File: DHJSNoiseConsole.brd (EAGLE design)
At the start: 88.9 x 34 mm, 11 parts

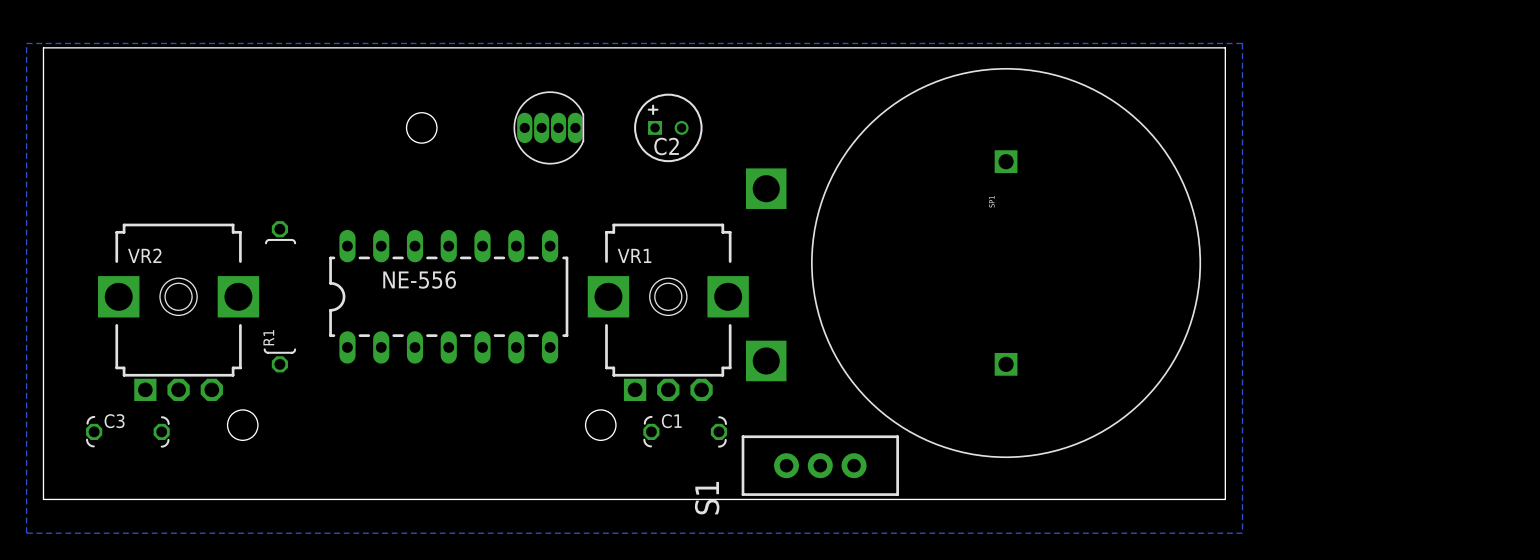
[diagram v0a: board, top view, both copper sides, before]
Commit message: board
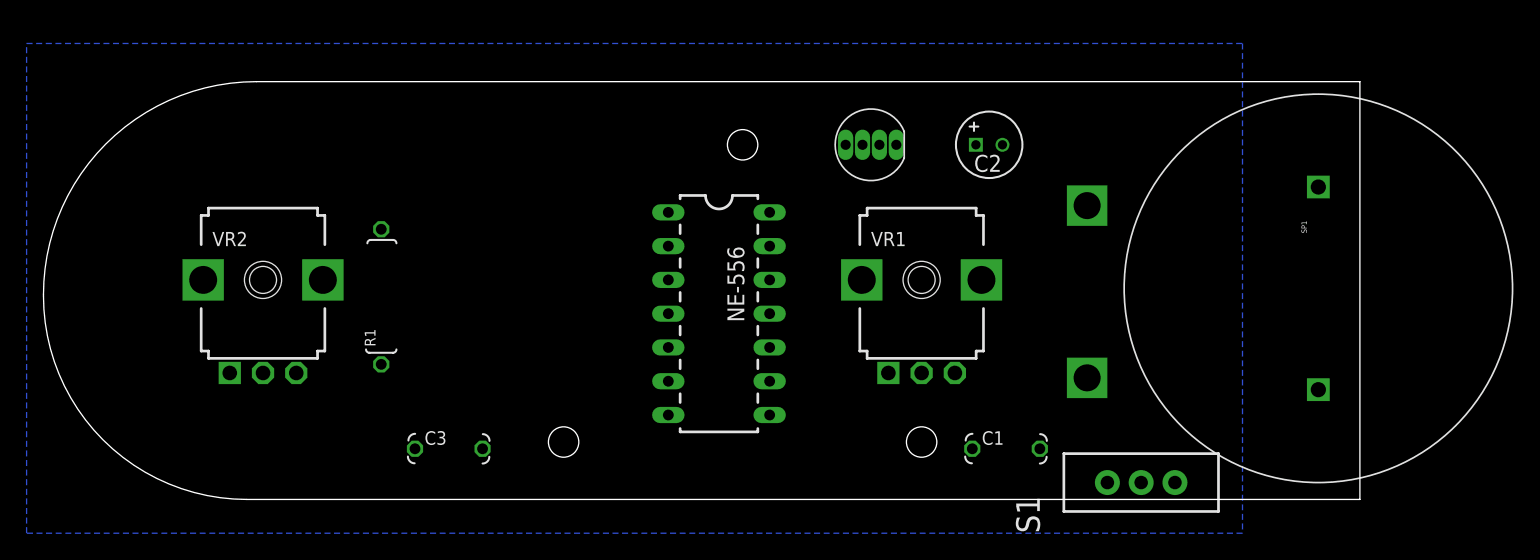
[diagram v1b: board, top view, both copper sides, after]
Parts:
- moved C1 24.2 mm to (72.4, 3.81)
- moved C2 24.2 mm to (71.1, 26.7)
- moved C3 24.2 mm to (30.5, 3.81)
- moved BAT1 24.2 mm to (25.4, 30.5)
- moved D1 24.2 mm to (62.2, 26.7)
- moved S1 24.2 mm to (82.5, 1.27)
- moved SP1 23.6 mm to (95.9, 15.9)
- moved NE-556 19.2 mm to (50.8, 12.7), turned to 270 degrees
- moved VR1 19.1 mm to (66.0, 16.5)
- moved R1 7.62 mm to (25.4, 15.2)
- moved VR2 6.48 mm to (16.5, 16.5)
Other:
- board size 88.9 x 34 mm -> 99 x 31.4 mm
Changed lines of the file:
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@@
 <setting verticaltext="up"/>
 </settings>
-<grid distance="0.05" unitdist="inch" unit="inch" style="lines" multiple="1" display="no" altdistance="0.025" altunitdist="inch" altunit="inch"/>
+<grid distance="0.05" unitdist="inch" unit="mm" style="lines" multiple="1" display="no" altdistance="0.025" altunitdist="inch" altunit="inch"/>
 <layers>
 <layer number="1" name="Top" color="4" fill="1" visible="yes" active="yes"/>
@@
 <board>
 <plain>
-<wire x1="0" y1="0" x2="88.88" y2="0" width="0" layer="20"/>
-<wire x1="88.88" y1="0" x2="88.88" y2="33.96" width="0" layer="20"/>
-<wire x1="88.88" y1="33.96" x2="0" y2="33.96" width="0" layer="20"/>
-<wire x1="0" y1="33.96" x2="0" y2="0" width="0" layer="20"/>
+<wire x1="99" y1="31.42" x2="16.007575" y2="31.42" width="0" layer="20"/>
+<wire x1="16.007575" y1="31.42" x2="0" y2="15.412425" width="0" layer="20" curve="90"/>
+<wire x1="0" y1="15.412425" x2="0" y2="15.292825" width="0" layer="20"/>
+<wire x1="0" y1="15.292825" x2="15.292825" y2="0" width="0" layer="20" curve="90"/>
+<wire x1="15.292825" y1="0" x2="99" y2="0" width="0" layer="20"/>
+<wire x1="99" y1="0" x2="99" y2="31.42" width="0" layer="20"/>
 </plain>
 <attributes>
@@
 </autorouter>
 <elements>
-<element name="BAT1" library="SparkFun-Connectors" package="BC9VPC" value="" x="1.27" y="31.75" rot="MR180">
-<attribute name="PROD_ID" value="BATT-10855" x="1.27" y="31.75" size="1.778" layer="28" rot="MR180" display="off"/>
+<element name="BAT1" library="SparkFun-Connectors" package="BC9VPC" value="" x="25.4" y="30.48" rot="MR180">
+<attribute name="PROD_ID" value="BATT-10855" x="25.4" y="30.48" size="1.778" layer="28" rot="MR180" display="off"/>
 </element>
-<element name="C1" library="TomW" package="C050-024X044" value="100n" x="48.26" y="5.08"/>
-<element name="C2" library="gm-caps-electro-pol" package="050_020" value="10uf" x="46.99" y="27.94"/>
-<element name="C3" library="TomW" package="C050-024X044" value="100n" x="6.35" y="5.08"/>
-<element name="NE-556" library="SparkFun-AnalogIC" package="DIL14" value="" x="31.75" y="15.24"/>
-<element name="R1" library="MusicThingModular" package="10MM_RESISTOR" value="1k" x="17.78" y="15.24" rot="R90"/>
-<element name="S1" library="SparkFun-Electromechanical" package="SWITCH-SPDT" value="" x="58.42" y="2.54" rot="R90"/>
-<element name="SP1" library="SparkFun-Electromechanical" package="PCB_MOUNT_SPEAKER" value="SPEAKERPCB_MOUNT" x="72.39" y="17.78" rot="R270">
-<attribute name="SPARKLE_ID" value="6504" x="72.39" y="17.78" size="1.778" layer="27" rot="R270" display="off"/>
-<attribute name="SKU" value="COM-11089" x="72.39" y="17.78" size="1.778" layer="27" rot="R270" display="off"/>
-<attribute name="MFG" value="SANCO" x="72.39" y="17.78" size="1.778" layer="27" rot="R270" display="off"/>
-<attribute name="PROD_#" value="NA" x="72.39" y="17.78" size="1.778" layer="27" rot="R270" display="off"/>
+<element name="C1" library="TomW" package="C050-024X044" value="100n" x="72.39" y="3.81"/>
+<element name="C2" library="gm-caps-electro-pol" package="050_020" value="10uf" x="71.12" y="26.67"/>
+<element name="C3" library="TomW" package="C050-024X044" value="100n" x="30.48" y="3.81"/>
+<element name="NE-556" library="SparkFun-AnalogIC" package="DIL14" value="" x="50.8" y="12.7" rot="R270"/>
+<element name="R1" library="MusicThingModular" package="10MM_RESISTOR" value="1k" x="25.4" y="15.24" rot="R90"/>
+<element name="S1" library="SparkFun-Electromechanical" package="SWITCH-SPDT" value="" x="82.55" y="1.27" rot="R90"/>
+<element name="SP1" library="SparkFun-Electromechanical" package="PCB_MOUNT_SPEAKER" value="SPEAKERPCB_MOUNT" x="95.875" y="15.875" rot="R270">
+<attribute name="SPARKLE_ID" value="6504" x="95.875" y="15.875" size="1.778" layer="27" rot="R270" display="off"/>
+<attribute name="SKU" value="COM-11089" x="95.875" y="15.875" size="1.778" layer="27" rot="R270" display="off"/>
+<attribute name="MFG" value="SANCO" x="95.875" y="15.875" size="1.778" layer="27" rot="R270" display="off"/>
+<attribute name="PROD_#" value="NA" x="95.875" y="15.875" size="1.778" layer="27" rot="R270" display="off"/>
 </element>
-<element name="VR1" library="MusicThingModular" package="9MM_SNAP-IN_POT" value="100k" x="46.99" y="15.24"/>
-<element name="VR2" library="MusicThingModular" package="9MM_SNAP-IN_POT" value="100k" x="10.16" y="15.24"/>
-<element name="D1" library="SparkFun-LED" package="LED-RGB-THRU" value="LED-RGB-CC-THRUCLEAR" x="38.1" y="27.94">
-<attribute name="PROD_ID" value="DIO-08418" x="38.1" y="27.94" size="1.778" layer="27" display="off"/>
+<element name="VR1" library="MusicThingModular" package="9MM_SNAP-IN_POT" value="100k" x="66.04" y="16.51"/>
+<element name="VR2" library="MusicThingModular" package="9MM_SNAP-IN_POT" value="100k" x="16.51" y="16.51"/>
+<element name="D1" library="SparkFun-LED" package="LED-RGB-THRU" value="LED-RGB-CC-THRUCLEAR" x="62.23" y="26.67">
+<attribute name="PROD_ID" value="DIO-08418" x="62.23" y="26.67" size="1.778" layer="27" display="off"/>
 </element>
 </elements>
@@
 <contactref element="VR2" pad="3"/>
 <contactref element="D1" pad="3"/>
-<wire x1="49.49" y1="8.24" x2="55.88" y2="2.54" width="0" layer="19" extent="1-1"/>
-<wire x1="30.48" y1="11.43" x2="49.49" y2="8.24" width="0" layer="19" extent="1-1"/>
-<wire x1="33.02" y1="19.05" x2="30.48" y2="11.43" width="0" layer="19" extent="1-1"/>
-<wire x1="37.465" y1="27.94" x2="33.02" y2="19.05" width="0" layer="19" extent="1-1"/>
-<wire x1="22.86" y1="19.05" x2="33.02" y2="19.05" width="0" layer="19" extent="1-1"/>
-<wire x1="12.66" y1="8.24" x2="22.86" y2="19.05" width="0" layer="19" extent="1-1"/>
+<wire x1="68.54" y1="9.51" x2="80.01" y2="1.27" width="0" layer="19" extent="1-1"/>
+<wire x1="46.99" y1="13.97" x2="68.54" y2="9.51" width="0" layer="19" extent="1-1"/>
+<wire x1="54.61" y1="11.43" x2="46.99" y2="13.97" width="0" layer="19" extent="1-1"/>
+<wire x1="61.595" y1="26.67" x2="54.61" y2="11.43" width="0" layer="19" extent="1-1"/>
+<wire x1="54.61" y1="21.59" x2="54.61" y2="11.43" width="0" layer="19" extent="1-1"/>
+<wire x1="19.01" y1="9.51" x2="54.61" y2="21.59" width="0" layer="19" extent="1-1"/>
 </signal>
 <signal name="N$1">
@@
 <contactref element="NE-556" pad="1"/>
 <contactref element="R1" pad="2"/>
-<wire x1="22.86" y1="11.43" x2="46.99" y2="8.24" width="0" layer="19" extent="1-1"/>
-<wire x1="17.78" y1="20.32" x2="22.86" y2="11.43" width="0" layer="19" extent="1-1"/>
+<wire x1="46.99" y1="21.59" x2="66.04" y2="9.51" width="0" layer="19" extent="1-1"/>
+<wire x1="25.4" y1="20.32" x2="46.99" y2="21.59" width="0" layer="19" extent="1-1"/>
 </signal>
 <signal name="N$2">
 <contactref element="S1" pad="2"/>
 <contactref element="BAT1" pad="V+"/>
-<wire x1="58.42" y1="2.54" x2="54.356" y2="10.414" width="0" layer="19" extent="1-1"/>
+<wire x1="82.55" y1="1.27" x2="78.486" y2="9.144" width="0" layer="19" extent="1-1"/>
 </signal>
 <signal name="GND">
@@
 <contactref element="SP1" pad="+"/>
 <contactref element="C2" pad="+"/>
-<wire x1="45.99" y1="27.94" x2="72.39" y2="25.4" width="0" layer="19" extent="1-1"/>
+<wire x1="70.12" y1="26.67" x2="95.875" y2="23.495" width="0" layer="19" extent="1-1"/>
 </signal>
 <signal name="N$6">
@@
 <contactref element="NE-556" pad="6"/>
 <contactref element="C1" pad="2"/>
-<wire x1="35.56" y1="11.43" x2="50.8" y2="5.08" width="0" layer="19" extent="1-1"/>
-<wire x1="25.4" y1="11.43" x2="35.56" y2="11.43" width="0" layer="19" extent="1-1"/>
-<wire x1="17.78" y1="10.16" x2="25.4" y2="11.43" width="0" layer="19" extent="1-1"/>
+<wire x1="46.99" y1="8.89" x2="74.93" y2="3.81" width="0" layer="19" extent="1-1"/>
+<wire x1="46.99" y1="19.05" x2="46.99" y2="8.89" width="0" layer="19" extent="1-1"/>
+<wire x1="25.4" y1="10.16" x2="46.99" y2="19.05" width="0" layer="19" extent="1-1"/>
 </signal>
 <signal name="N$3">
@@
 <contactref element="NE-556" pad="12"/>
 <contactref element="C3" pad="1"/>
-<wire x1="25.4" y1="19.05" x2="27.94" y2="19.05" width="0" layer="19" extent="1-1"/>
-<wire x1="10.16" y1="8.24" x2="25.4" y2="19.05" width="0" layer="19" extent="1-1"/>
-<wire x1="3.81" y1="5.08" x2="10.16" y2="8.24" width="0" layer="19" extent="1-1"/>
+<wire x1="54.61" y1="19.05" x2="54.61" y2="16.51" width="0" layer="19" extent="1-1"/>
+<wire x1="16.51" y1="9.51" x2="54.61" y2="19.05" width="0" layer="19" extent="1-1"/>
+<wire x1="27.94" y1="3.81" x2="16.51" y2="9.51" width="0" layer="19" extent="1-1"/>
 </signal>
 <signal name="R">
@@
 <contactref element="NE-556" pad="9"/>
 <contactref element="C2" pad="-"/>
-<wire x1="40.005" y1="27.94" x2="47.99" y2="27.94" width="0" layer="19" extent="1-1"/>
-<wire x1="35.56" y1="19.05" x2="40.005" y2="27.94" width="0" layer="19" extent="1-1"/>
+<wire x1="64.135" y1="26.67" x2="72.12" y2="26.67" width="0" layer="19" extent="1-1"/>
+<wire x1="54.61" y1="8.89" x2="64.135" y2="26.67" width="0" layer="19" extent="1-1"/>
 </signal>
 <signal name="B">
@@
 <contactref element="NE-556" pad="5"/>
 <contactref element="NE-556" pad="8"/>
-<wire x1="38.1" y1="19.05" x2="36.195" y2="27.94" width="0" layer="19" extent="1-1"/>
-<wire x1="33.02" y1="11.43" x2="38.1" y2="19.05" width="0" layer="19" extent="1-1"/>
+<wire x1="54.61" y1="6.35" x2="60.325" y2="26.67" width="0" layer="19" extent="1-1"/>
+<wire x1="46.99" y1="11.43" x2="54.61" y2="6.35" width="0" layer="19" extent="1-1"/>
 </signal>
 </signals>

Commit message: board
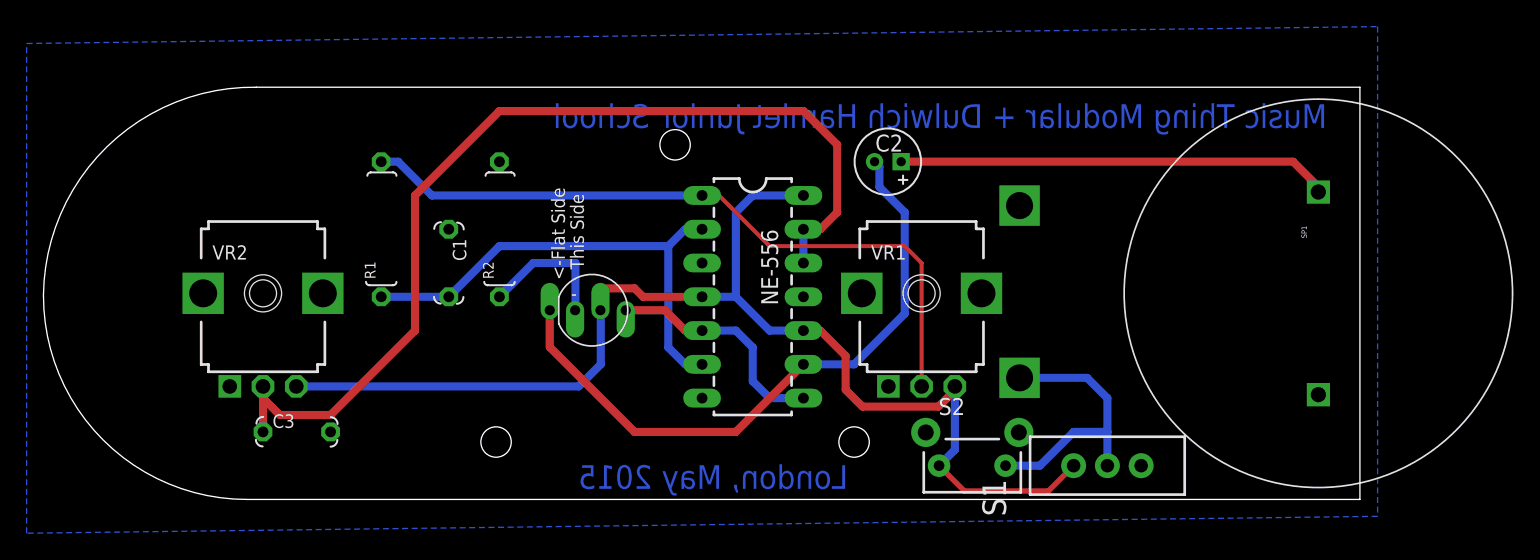
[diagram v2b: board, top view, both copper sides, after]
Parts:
- added R2: 2k, MusicThingModular:10MM_RESISTOR
- added S2: (no value), SparkFun-Electromechanical:TACTILE-PTH-SIDEEZ
- added U$1: (no value), TW_logos:MTM_1CM_KEEPOUT
- moved C1 44.2 mm to (30.5, 17.8), turned to 270 degrees
- moved D1 24.4 mm to (41.2, 14.2), turned to 180 degrees
- moved C3 11.5 mm to (19.1, 5.08)
- moved C2 7.73 mm to (63.5, 25.4), turned to 180 degrees
- moved R1 5.08 mm to (25.4, 20.3)
- moved BAT1 5.08 mm to (20.3, 30.5)
- moved NE-556 2.84 mm to (53.3, 14.0)
- moved S1 2.84 mm to (80.0, 2.54)
- moved VR1 1.01 mm to (66.0, 15.5)
- moved VR2 1.01 mm to (16.5, 15.5)
- moved SP1 0.38 mm to (95.9, 15.5)
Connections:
- new net N$4: D1.2, R2.1
- net +9V: now also S2.1
- net GND: now also R2.2; no longer D1.2
- net N$2: now also S2.2
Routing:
- net +9V: track 0.00 -> 92.0 mm
- net N$3: track 0.00 -> 75.2 mm
- net N$1: track 0.00 -> 53.1 mm
- net R: track 0.00 -> 48.2 mm
- net N$6: track 0.00 -> 36.9 mm
- net N$7: track 0.00 -> 32.5 mm
- net N$2: track 0.00 -> 21.0 mm
- net B: track 0.00 -> 17.6 mm
- net N$4: track 0.00 -> 10.3 mm
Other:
- board size 99 x 31.4 mm -> 99 x 31 mm
- board text added: "-"
- board text added: "<-Flat Side This Side"
- board text added: "London, May 2015"
- board text added: "Music Thing Modular + Dulwich Hamlet Junior School"
